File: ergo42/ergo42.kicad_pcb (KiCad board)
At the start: 2 copper layers, 135.9 x 102.2 mm, 69 parts, among them J1 5PIN, SW1 SW_PUSH, SW10 SW_PUSH, SW11 SW_PUSH, SW12 SW_PUSH, SW13 SW_PUSH, SW14 SW_PUSH, SW15 SW_PUSH, SW16 SW_PUSH, SW17 SW_PUSH, SW18 SW_PUSH, SW19 SW_PUSH, SW2 SW_PUSH, SW20 SW_PUSH, SW21 SW_PUSH, SW22 SW_PUSH, SW23 SW_PUSH, SW24 SW_PUSH, SW25 SW_PUSH, SW26 SW_PUSH, SW27 SW_PUSH, SW28 SW_PUSH, SW29 SW_Push, SW3 SW_PUSH, SW4 SW_PUSH, SW5 SW_PUSH, SW6 SW_PUSH, SW7 SW_PUSH, SW8 SW_PUSH, SW9 SW_PUSH, U1 HOLE, U2 HOLE, U3 ProMicro, U4 HOLE, U5 HOLE, U7 HOLE

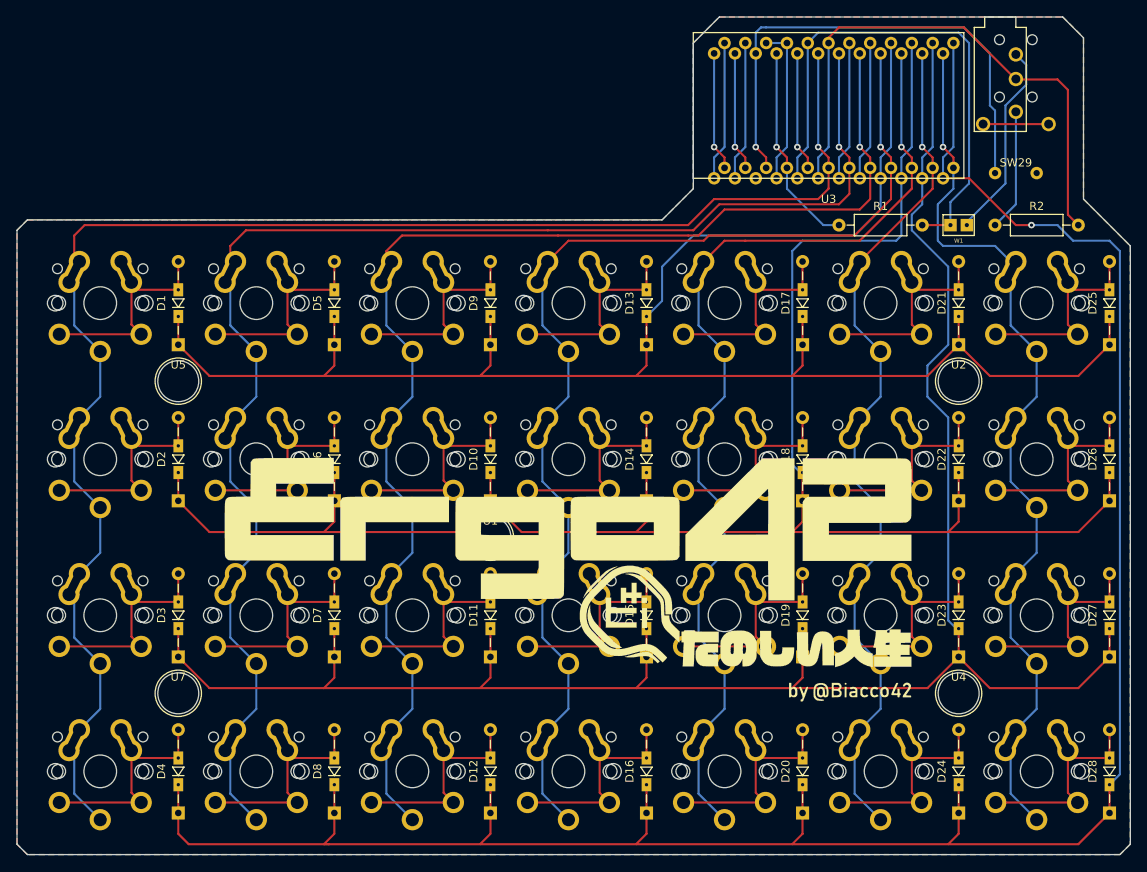
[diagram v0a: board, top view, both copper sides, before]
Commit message: hot swap
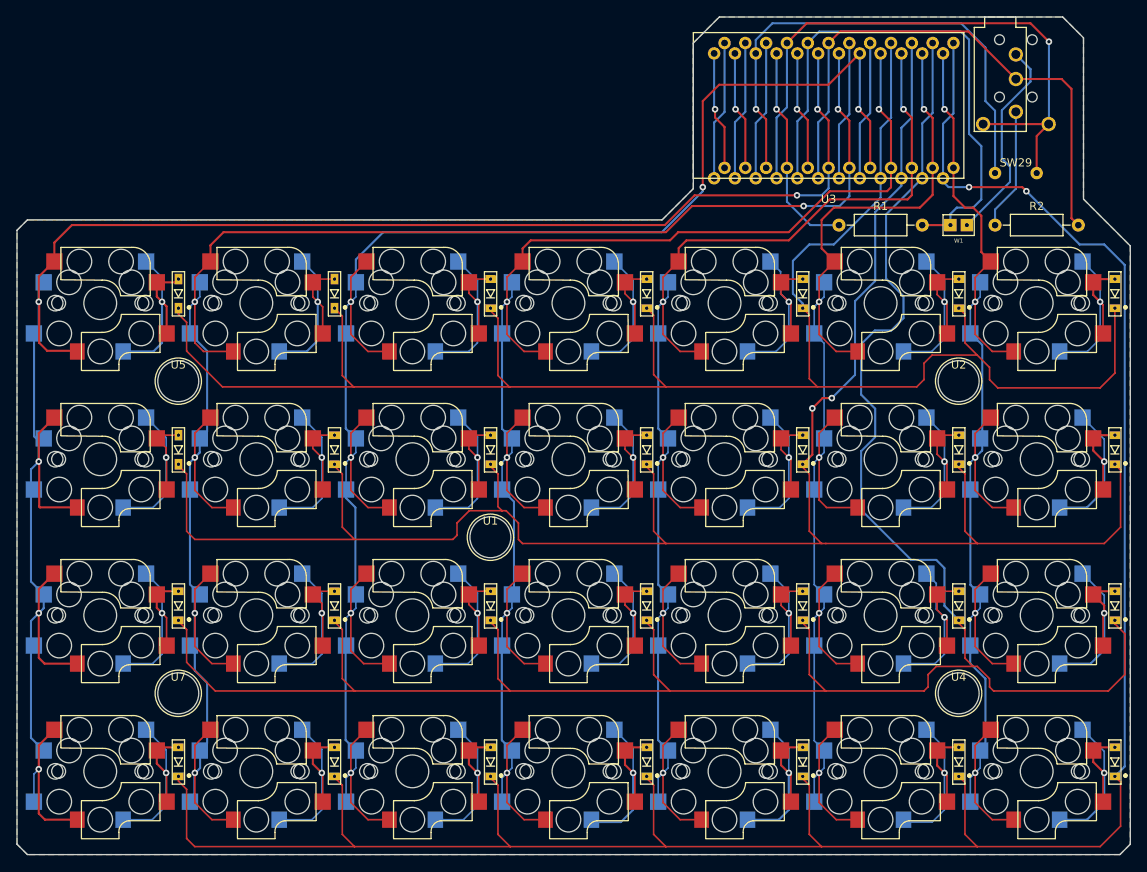
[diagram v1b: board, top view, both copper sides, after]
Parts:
- removed G*** (x2): LOGO, library:ergo42_logo
- D1, D10, D11, D12, D13, D14, D15, D16, D17, D18, D19, D2, D20, D21, D22, D23, D24, D25, D26, D27, D28, D3, D4, D5, D6, D7, D8, D9: footprint library:Diode_SMD_THT -> library:Diode_TH
- SW1, SW10, SW11, SW12, SW13, SW14, SW15, SW16, SW17, SW18, SW19, SW2, SW20, SW21, SW22, SW23, SW24, SW25, SW26, SW27, SW28, SW3, SW4, SW5, SW6, SW7, SW8, SW9: footprint library:key_switch -> library:CherryMX_Choc_Hotswap
- moved D10 6.76 mm to (131.6, 91.0), turned to 0 degrees
- moved D11 6.76 mm to (131.6, 110.1), turned to 0 degrees
- moved D18 6.76 mm to (169.7, 91.0), turned to 0 degrees
- moved D19 6.76 mm to (169.7, 110.1), turned to 0 degrees
- moved D14 6.76 mm to (150.7, 91.0), turned to 0 degrees
- moved D15 6.76 mm to (150.7, 110.1), turned to 0 degrees
- moved D2 6.76 mm to (93.5, 91.0), turned to 0 degrees
- moved D22 6.76 mm to (188.8, 91.0), turned to 0 degrees
- moved D23 6.76 mm to (188.8, 110.1), turned to 0 degrees
- moved D3 6.76 mm to (93.5, 110.1), turned to 0 degrees
- moved D6 6.76 mm to (112.5, 91.0), turned to 0 degrees
- moved D7 6.76 mm to (112.5, 110.1), turned to 0 degrees
- moved D1 6.76 mm to (93.5, 72.0), turned to 0 degrees
- moved D17 6.76 mm to (169.7, 72.0), turned to 0 degrees
- moved D5 6.76 mm to (112.5, 72.0), turned to 0 degrees
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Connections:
- net /scl/uart renamed /scl/uart
- U3 pad 1: Net-(U3-Pad1) -> unconnected-(U3-TX-Pad1)
- U3 pad 2: Net-(U3-Pad2) -> unconnected-(U3-RX-Pad2)_1
- U3 pad 20: Net-(U3-Pad20) -> unconnected-(U3-F4-Pad20)_1
- U3 pad 24: Net-(U3-Pad24) -> unconnected-(U3-RAW-Pad24)_1
- U3 pad 7: Net-(U3-Pad7) -> unconnected-(U3-D4-Pad7)_1
- U3 pad 8: Net-(U3-Pad8) -> unconnected-(U3-C6-Pad8)_1
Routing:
- net (no net): track 0.00 -> 97.2 mm, vias 0 -> 2
- net /col2: track 158.3 -> 224.3 mm, vias 1 -> 6
- net GND: track 42.1 -> 107.1 mm, vias 1 -> 2
- net /col5: track 106.8 -> 169.1 mm, vias 1 -> 5
- net /col0: track 191.6 -> 249.0 mm, vias 1 -> 6
- net /col1: track 174.8 -> 229.4 mm, vias 1 -> 6
- net /col3: track 141.2 -> 194.8 mm, vias 1 -> 5
- net /col4: track 126.2 -> 178.5 mm, vias 1 -> 5
- net /col6: track 111.1 -> 157.1 mm, vias 1 -> 5
- net /row2: track 239.0 -> 263.8 mm
- net Net-(U3-Pad8): track 17.0 -> 0.00 mm
- net Net-(U3-Pad7): track 17.0 -> 0.00 mm
- net Net-(U3-Pad1): track 17.0 -> 0.00 mm
- net Net-(U3-Pad2): track 17.0 -> 0.00 mm
- net /row1: track 227.3 -> 242.9 mm, vias 0 -> 2
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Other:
- net class Default removed
